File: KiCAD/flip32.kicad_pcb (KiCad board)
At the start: 2 copper layers, 36 x 36 mm, 60 parts, among them CON1 USB, IC2 MIC5205, Q1 MMBT29, U1 LP38691, U2 MPU-9250, U3 STM32F103CB, U5 MS5611-01BA, U6 CP2102, X1 8MHZ

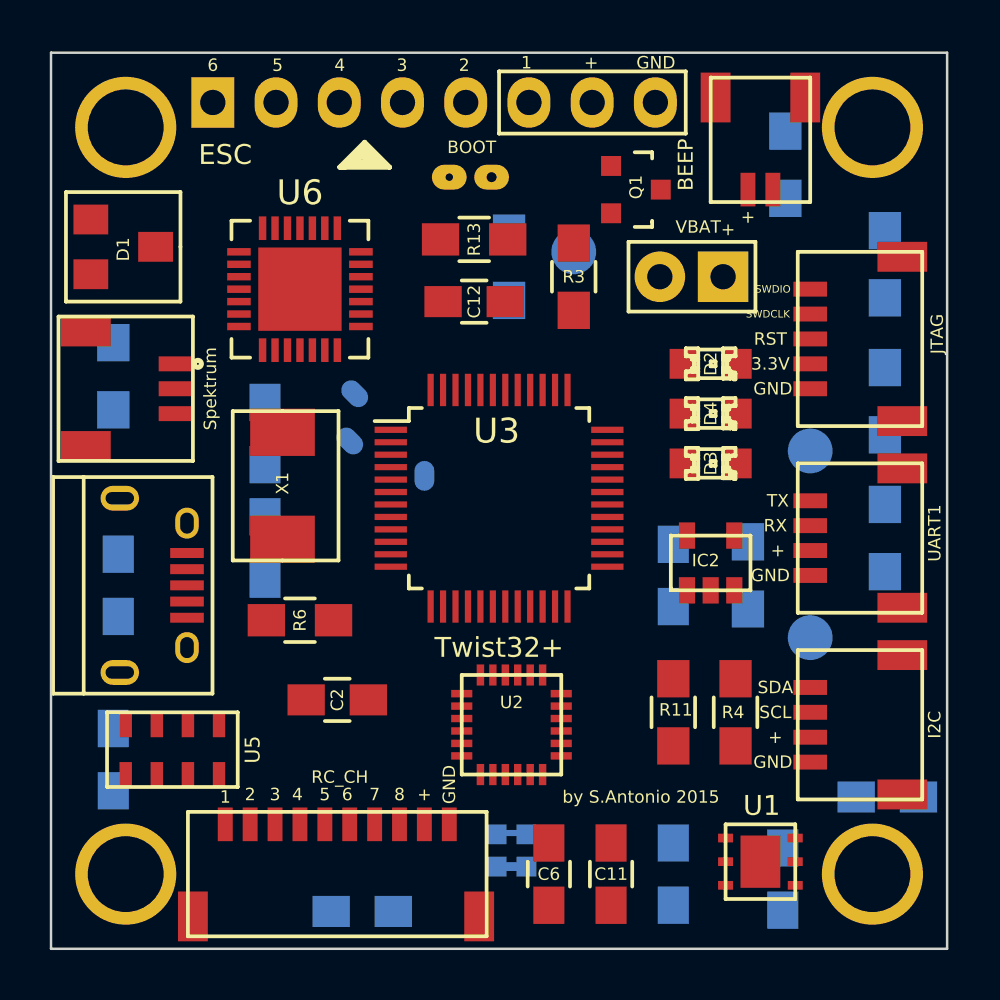
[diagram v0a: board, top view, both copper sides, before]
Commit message: pcb completed
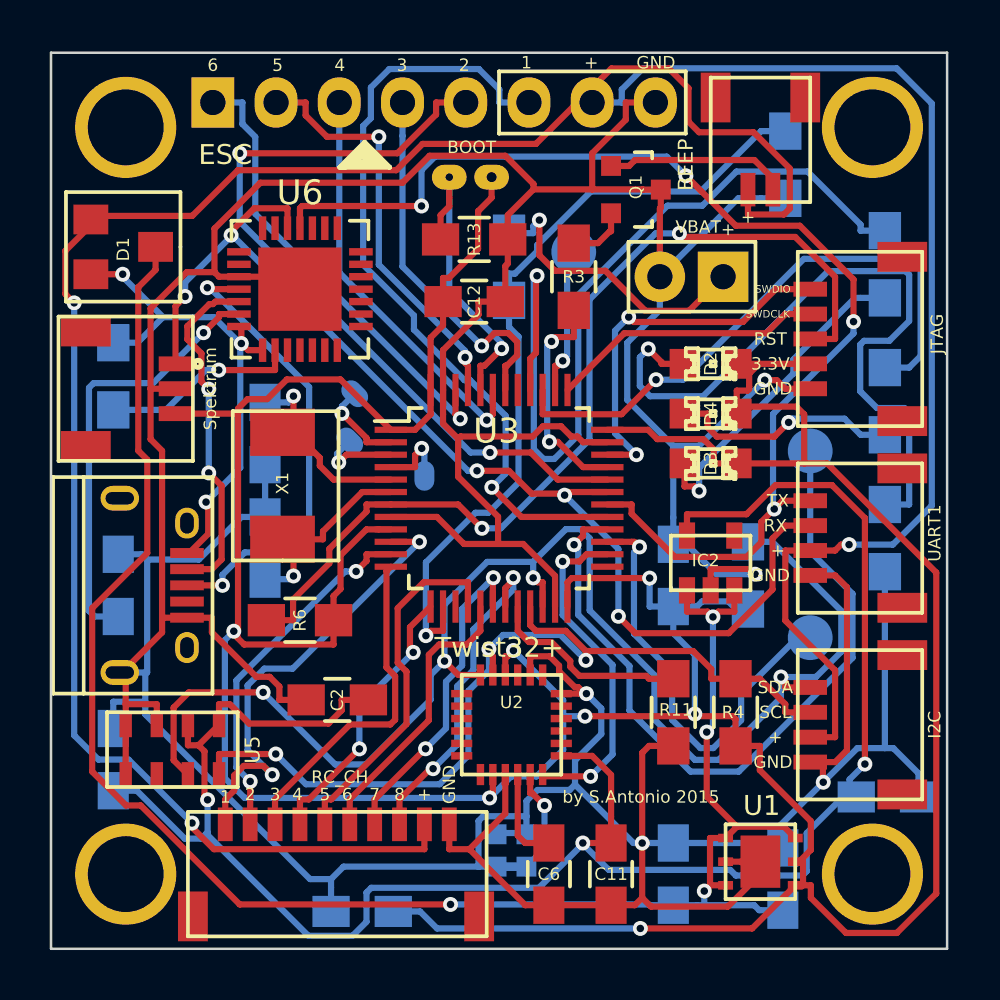
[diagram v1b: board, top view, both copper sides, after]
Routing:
- net GND: track 0.00 -> 250.2 mm, vias 0 -> 5
- net VCC: track 0.00 -> 163.9 mm, vias 0 -> 7
- net /VCC_IN: track 0.00 -> 124.0 mm, vias 0 -> 3
- net /VCC_SEN: track 0.00 -> 78.0 mm, vias 0 -> 3
- net /TO_REGS: track 0.00 -> 72.5 mm, vias 0 -> 4
- net /SDA: track 0.00 -> 57.7 mm, vias 0 -> 4
- net /TX0: track 0.00 -> 48.0 mm, vias 0 -> 4
- net /RX0: track 0.00 -> 46.0 mm, vias 0 -> 5
- net /NRST: track 0.00 -> 38.6 mm, vias 0 -> 2
- net /SCL: track 0.00 -> 36.3 mm, vias 0 -> 3
- net /LED0: track 0.00 -> 35.2 mm, vias 0 -> 1
- net /PWM2: track 0.00 -> 32.0 mm, vias 0 -> 2
- net /POWER_ADC: track 0.00 -> 31.9 mm, vias 0 -> 1
- net /PWM1: track 0.00 -> 31.6 mm, vias 0 -> 1
- net /UU8: track 0.00 -> 30.2 mm, vias 0 -> 1
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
